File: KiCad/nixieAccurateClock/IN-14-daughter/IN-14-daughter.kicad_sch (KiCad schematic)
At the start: 8 parts, among them J1 Conn_02x05_Odd_Even, U1 HV509K6-G

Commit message: Fill out BOM
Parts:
- C1, C2: Model (none) -> CL10B104KB8NNWC; Price (none) -> 0.10
- H1, H2: now left out of the parts list
- J1: Model (none) -> PPPC052LFBN-RC; Price (none) -> 0.72
- N1: Model (none) -> IN-14; Price (none) -> 17.50
- R1: Model (none) -> RC1206JR-0733KL; Price (none) -> 0.10
- U1: Price (none) -> 2.89
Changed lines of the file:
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@@
       (effects (font (size 1.27 1.27)) hide)
     )
-    (property "Datasheet" "~" (at 59.69 167.64 0)
+    (property "Datasheet" "https://mm.digikey.com/Volume0/opasdata/d220001/medias/docus/658/CL10B104KB8NNWC_Spec.pdf" (at 59.69 167.64 0)
+      (effects (font (size 1.27 1.27)) hide)
+    )
+    (property "Model" "CL10B104KB8NNWC" (at 59.69 167.64 0)
+      (effects (font (size 1.27 1.27)) hide)
+    )
+    (property "Price" "0.10" (at 59.69 167.64 0)
       (effects (font (size 1.27 1.27)) hide)
     )
@@
   )
   (symbol (lib_id "Mechanical:MountingHole_Pad") (at 137.16 24.13 0) (unit 1)
-    (in_bom yes) (on_board yes) (dnp no) (fields_autoplaced)
+    (in_bom no) (on_board yes) (dnp no) (fields_autoplaced)
     (property "Reference" "H1" (at 139.7 21.59 0)
       (effects (font (size 1.27 1.27)) (justify left))
@@
     )
   )
-  (symbol (lib_id "Device:C_Small") (at 74.93 167.64 0) (unit 1)
+  (symbol (lib_name "C_Small_1") (lib_id "Device:C_Small") (at 74.93 167.64 0) (unit 1)
     (in_bom yes) (on_board yes) (dnp no) (fields_autoplaced)
     (property "Reference" "C2" (at 77.47 166.3763 0)
@@
       (effects (font (size 1.27 1.27)) hide)
     )
-    (property "Datasheet" "~" (at 74.93 167.64 0)
+    (property "Datasheet" "https://mm.digikey.com/Volume0/opasdata/d220001/medias/docus/658/CL10B104KB8NNWC_Spec.pdf" (at 74.93 167.64 0)
+      (effects (font (size 1.27 1.27)) hide)
+    )
+    (property "Model" "CL10B104KB8NNWC" (at 74.93 167.64 0)
+      (effects (font (size 1.27 1.27)) hide)
+    )
+    (property "Price" "0.10" (at 74.93 167.64 0)
       (effects (font (size 1.27 1.27)) hide)
     )
@@
   )
   (symbol (lib_name "MountingHole_Pad_1") (lib_id "Mechanical:MountingHole_Pad") (at 166.37 24.13 0) (unit 1)
-    (in_bom yes) (on_board yes) (dnp no) (fields_autoplaced)
+    (in_bom no) (on_board yes) (dnp no) (fields_autoplaced)
     (property "Reference" "H2" (at 168.91 21.59 0)
       (effects (font (size 1.27 1.27)) (justify left))
@@
       (effects (font (size 0.508 0.508)) hide)
     )
-    (property "Datasheet" "" (at 71.12 46.99 0)
+    (property "Datasheet" "https://download.elektronicastynus.be/57/in-14_datasheet.pdf" (at 71.12 46.99 0)
+      (effects (font (size 1.27 1.27)) hide)
+    )
+    (property "Model" "IN-14" (at 71.12 46.99 90)
+      (effects (font (size 1.27 1.27)) hide)
+    )
+    (property "Price" "17.50" (at 71.12 46.99 90)
       (effects (font (size 1.27 1.27)) hide)
     )
@@
     (property "Datasheet" "https://ww1.microchip.com/downloads/en/DeviceDoc/hv509.pdf" (at 44.45 120.65 0)
       (effects (font (size 1.27 1.27) italic) hide)
+    )
+    (property "Price" "2.89" (at 92.71 93.98 90)
+      (effects (font (size 1.27 1.27)) hide)
     )
     (pin "27")
@@
       (effects (font (size 1.27 1.27)) hide)
     )
-    (property "Datasheet" "~" (at 73.66 29.21 0)
+    (property "Datasheet" "https://www.yageo.com/upload/media/product/app/datasheet/rchip/pyu-rc_group_51_rohs_l.pdf" (at 73.66 29.21 0)
+      (effects (font (size 1.27 1.27)) hide)
+    )
+    (property "Model" "RC1206JR-0733KL" (at 73.66 29.21 0)
+      (effects (font (size 1.27 1.27)) hide)
+    )
+    (property "Price" "0.10" (at 73.66 29.21 0)
       (effects (font (size 1.27 1.27)) hide)
     )
@@
       (effects (font (size 1.27 1.27)) hide)
     )
-    (property "Datasheet" "~" (at 148.59 64.77 0)
-      (effects (font (size 1.27 1.27)) hide)
-    )
+    (property "Datasheet" "https://mm.digikey.com/Volume0/opasdata/d220001/medias/docus/937/Female_Headers.100_DS.pdf" (at 148.59 64.77 0)
+      (effects (font (size 1.27 1.27)) hide)
+    )
+    (property "Model" "PPPC052LFBN-RC" (at 148.59 64.77 0)
+      (effects (font (size 1.27 1.27)) hide)
+    )
+    (property "Price" "0.72" (at 148.59 64.77 0)
+      (effects (font (size 1.27 1.27)) hide)
+    )

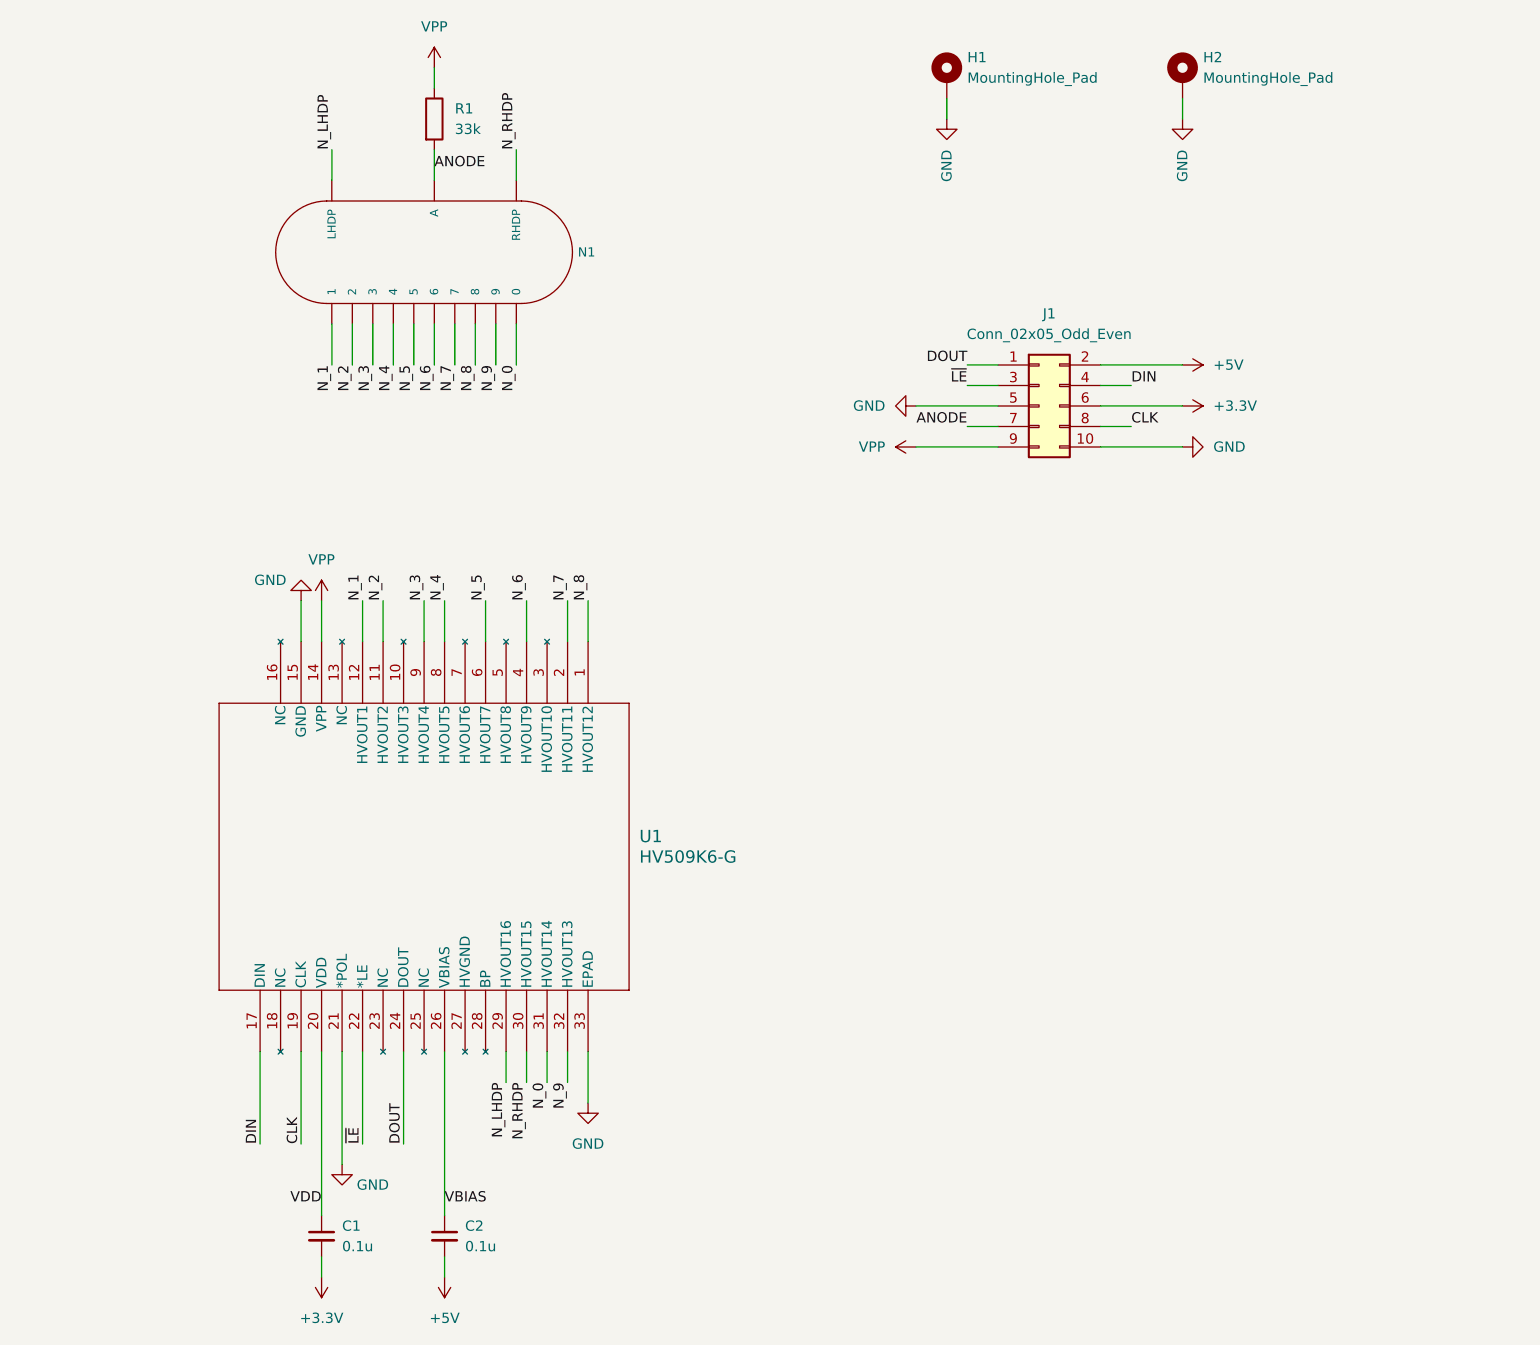
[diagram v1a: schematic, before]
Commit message: Add retailer links
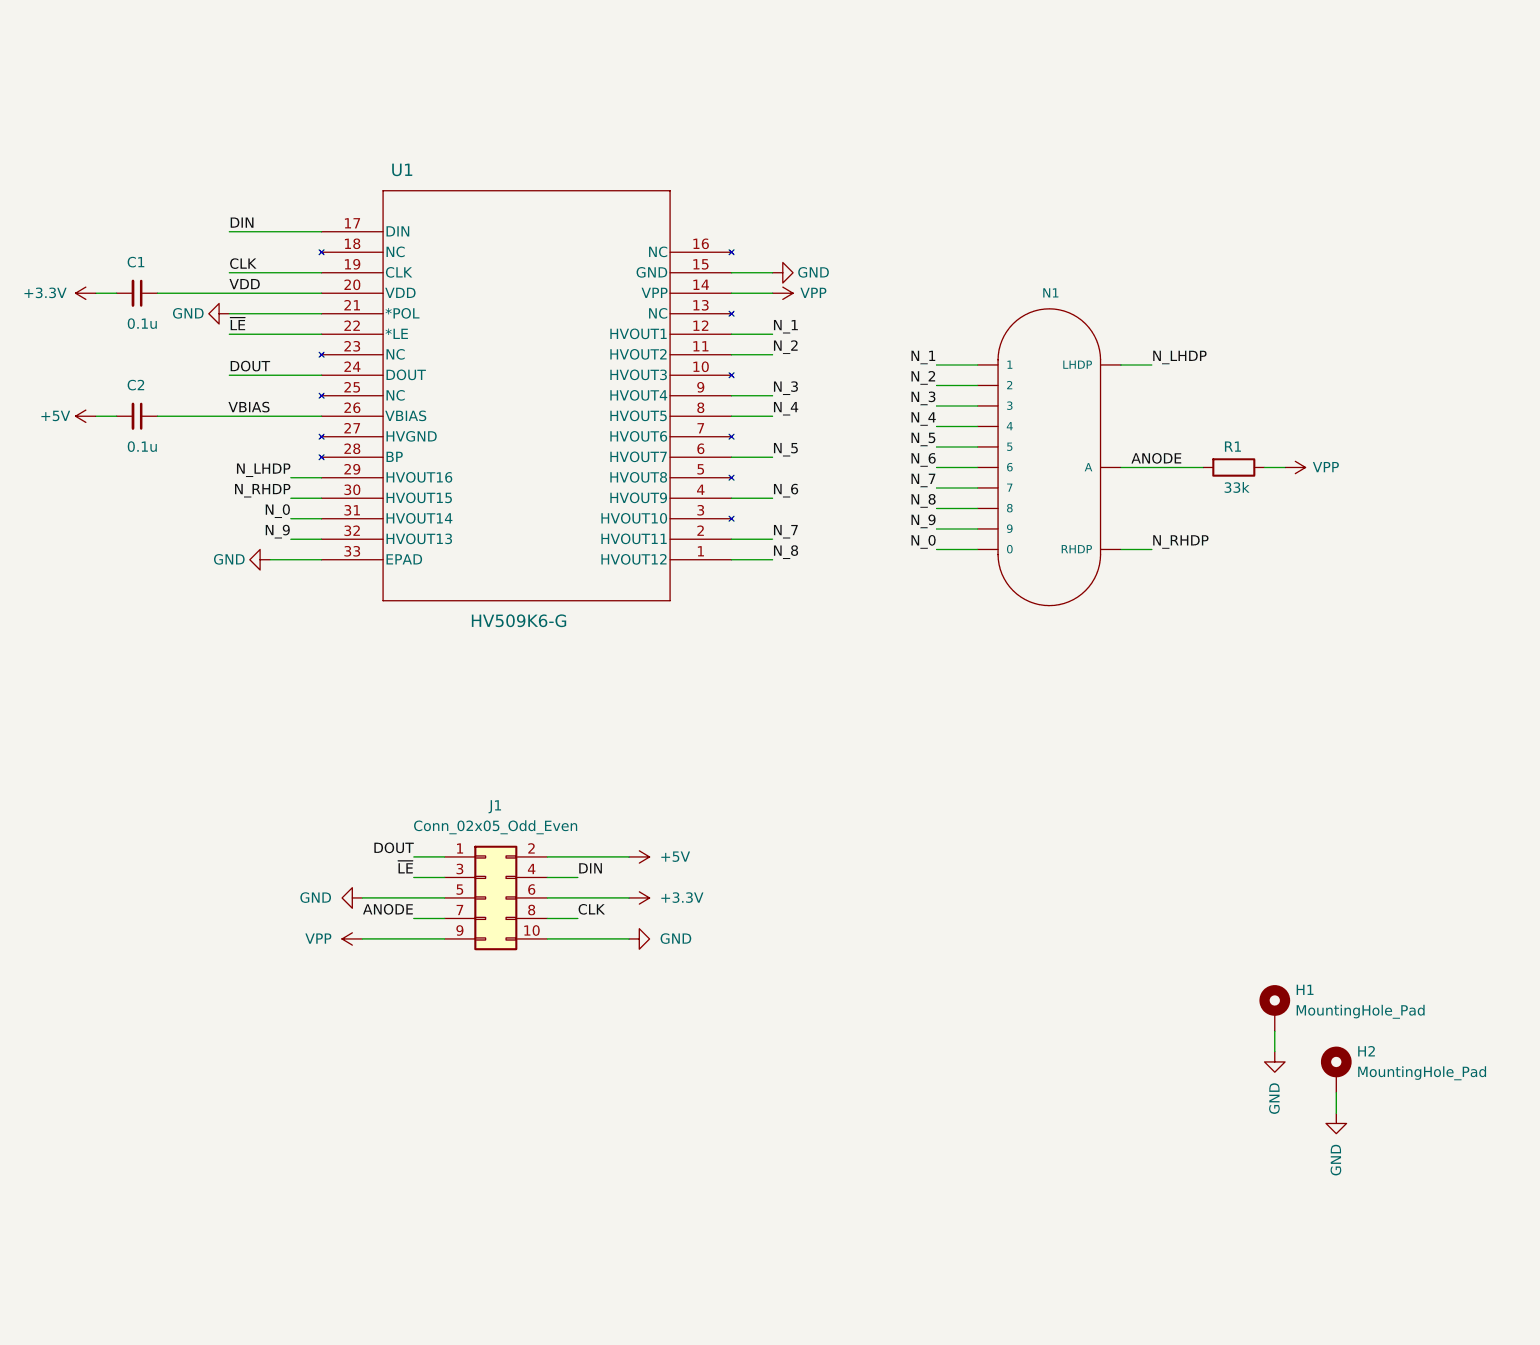
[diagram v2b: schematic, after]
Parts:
- C1, C2: Digikey link (none) -> https://www.digikey.com/en/products/detail/samsung-electro-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; Mouser link (none) -> https://www.mouser.com/ProductDetail/Samsung-Electro-Mechan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
- J1: Digikey link (none) -> https://www.digikey.com/en/products/detail/sullins-connecto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; Mouser link (none) -> N/A
- N1: Digikey link (none) -> N/A; Mouser link (none) -> N/A
- R1: Digikey link (none) -> https://www.digikey.com/en/products/detail/yageo/RC1206JR-0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; Mouser link (none) -> https://www.mouser.com/ProductDetail/YAGEO/RC1206JR-0733KL?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
- U1: Digikey link (none) -> https://www.digikey.com/en/products/detail/microchip-techno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; Model (none) -> HV509K6-G; Mouser link (none) -> https://www.mouser.com/ProductDetail/Microchip-Technology/H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
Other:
- moved on the sheet: C1, C2, H1, H2, J1, N1, R1, U1
